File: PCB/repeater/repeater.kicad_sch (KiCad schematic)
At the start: 34 parts, among them J2 RF_IN, U1 DRA818V, U2 DRA818U, U3 PGA-103

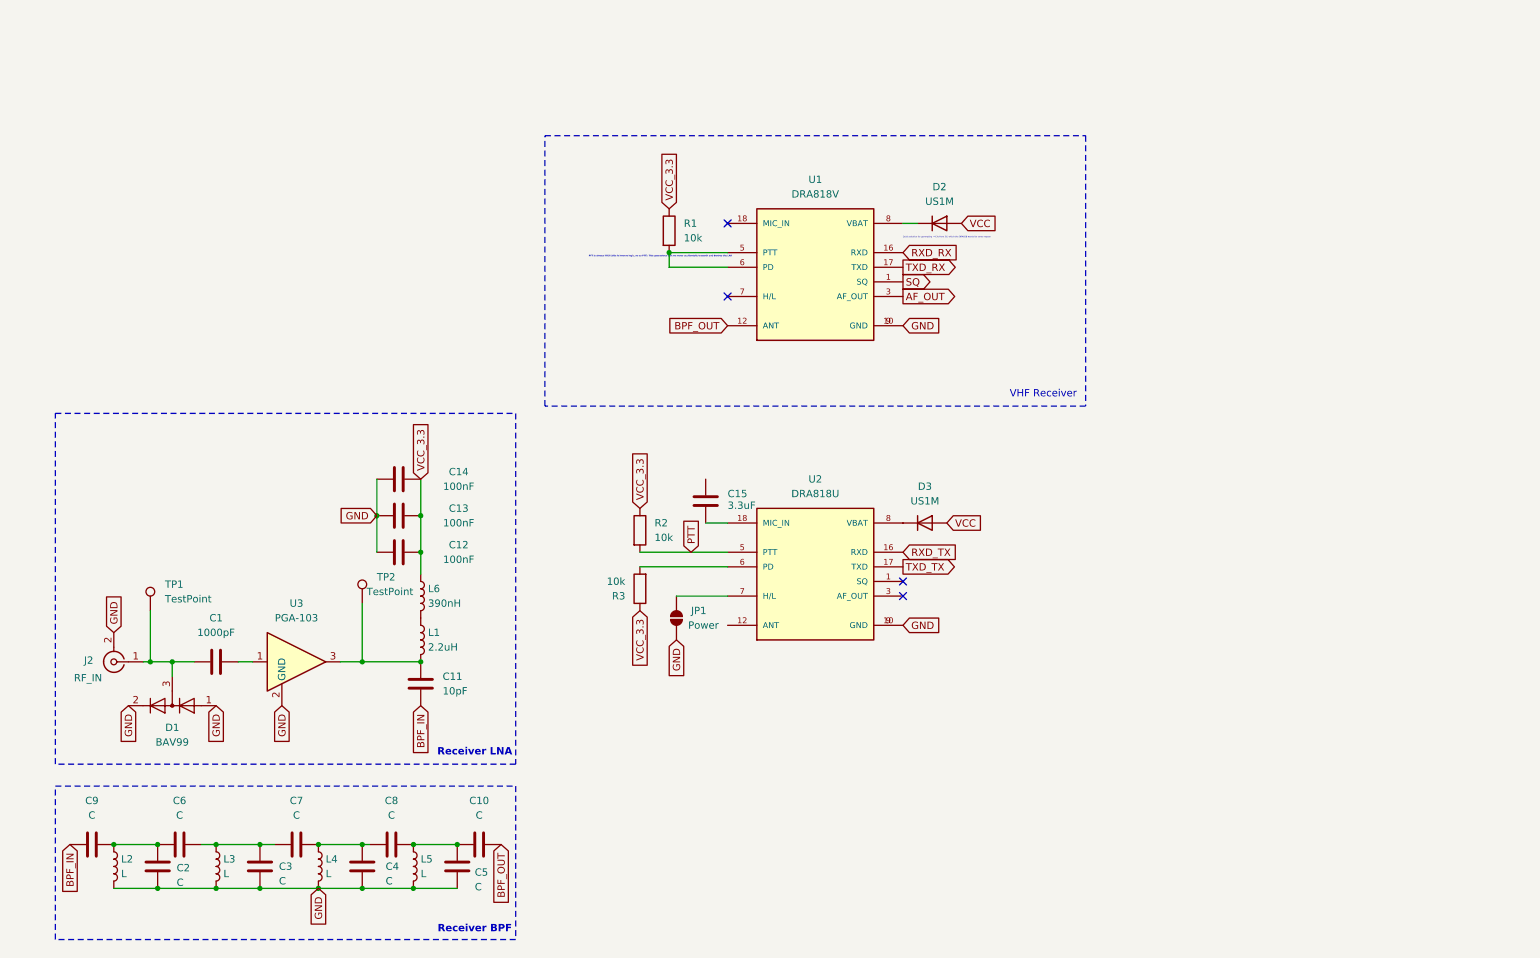
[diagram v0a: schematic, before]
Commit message: Continue routing
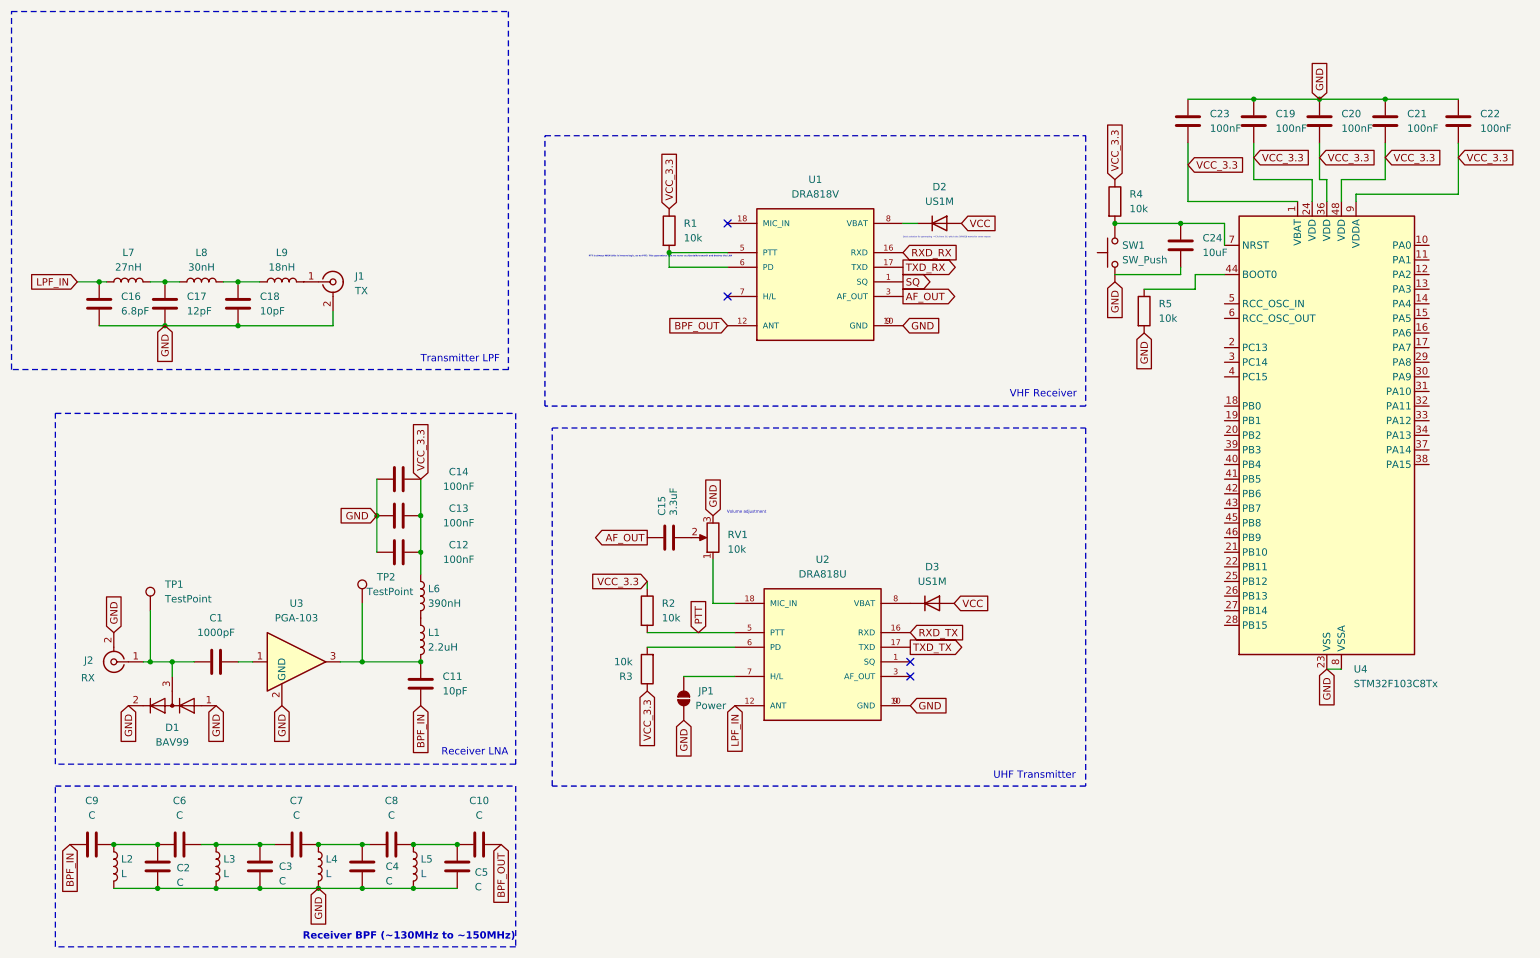
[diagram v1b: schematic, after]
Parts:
- added C16: 6.8pF, symbol Device:C
- added C17: 12pF, symbol Device:C
- added C18: 10pF, symbol Device:C
- added C19, C20, C21, C22, C23: 100nF, symbol Device:C
- added C24: 10uF, symbol Device:C
- added J1: TX, symbol Connector:Conn_Coaxial
- added L7: 27nH, symbol Device:L
- added L8: 30nH, symbol Device:L
- added L9: 18nH, symbol Device:L
- added R4: 10k, symbol Device:R
- added R5: 10k, Resistor_SMD:R_0603_1608Metric_Pad0.98x0.95mm_HandSolder, symbol Device:R
- added RV1: 10k, symbol Device:R_Potentiometer
- added SW1: SW_Push, symbol Switch:SW_Push
- added U4: STM32F103C8Tx, Package_QFP:LQFP-48_7x7mm_P0.5mm, symbol MCU_ST_STM32F1:STM32F103C8Tx
- J2: value RF_IN -> RX
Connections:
- net AF_OUT: now also C15.1
- net GND: now also C16.2, C17.2, C18.2, C19.1, C20.1, C21.1, C22.1, C23.1, J1.2 (Ext), R5.2, RV1.3, SW1.1, U4.23 (VSS), U4.35 (VSS), U4.47 (VSS), U4.8 (VSSA)
- net VCC_3.3: now also C19.2, C20.2, C21.2, C22.2, C23.2, R4.1, U4.1 (VBAT), U4.24 (VDD), U4.36 (VDD), U4.48 (VDD), U4.9 (VDDA)
- net LPF_IN: now reaches U2.12 (ANT)
- net LPF_IN: now also C16.1, L7.1
- net at U2.18 (MIC_IN): now also RV1.1; no longer C15.2
- new net: C24.1, R4.2, SW1.2, U4.7 (NRST)
- new net: C15.2, RV1.2
- new net: R5.1, U4.44 (BOOT0)
- new net: C18.1, L8.2, L9.1
- new net: C17.1, L7.2, L8.1
- new net: J1.1 (In), L9.2
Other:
- note added: "Receiver BPF (~130MHz to ~150MHz)"
- note added: "Transmitter LPF"
- note added: "UHF Transmitter"
- note added: "Volume adjustment"
- note removed: "Receiver BPF"
- moved on the sheet: C15, D3, JP1, R2, R3, U2
